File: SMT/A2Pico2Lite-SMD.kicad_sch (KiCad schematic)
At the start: 49 parts, among them J1 SolderJumper_2_Bridged, SW1 SW_BOOTSEL, U1 RP2354A-QFN60, U2 ME6211, X1 ABM8-272-T3 12MHz

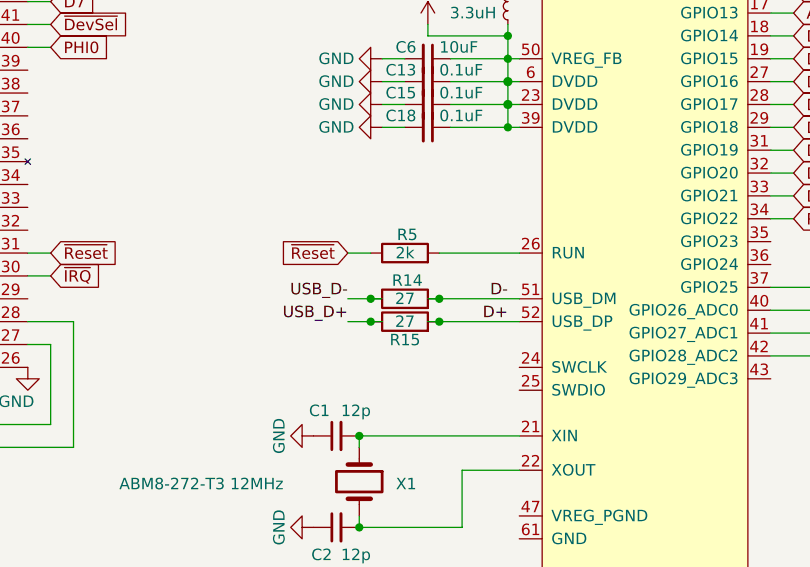
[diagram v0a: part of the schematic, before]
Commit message: Add files via upload
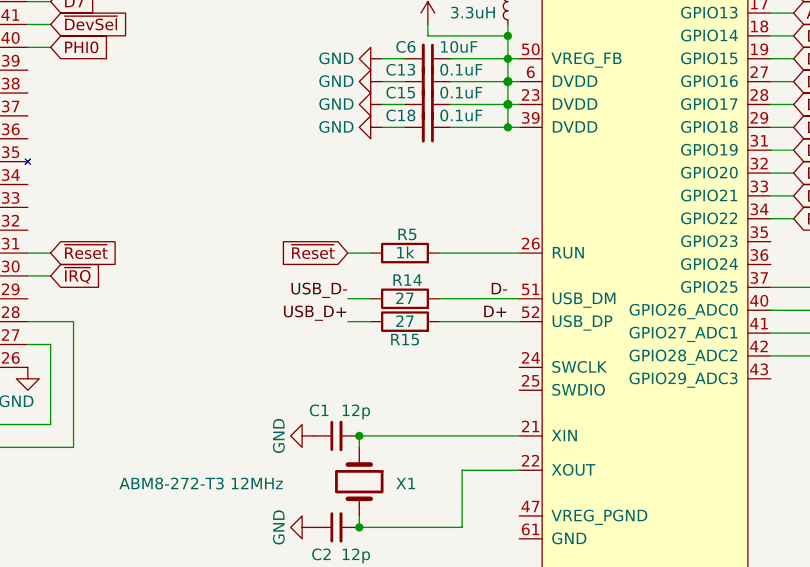
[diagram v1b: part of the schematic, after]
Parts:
- R5: value 2k -> 1k
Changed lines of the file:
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@@
 	)
 	(junction
-		(at 115.57 125.73)
-		(diameter 0)
-		(color 0 0 0 0)
-	)
-	(junction
-		(at 107.95 123.19)
-		(diameter 0)
-		(color 0 0 0 0)
-	)
-	(junction
 		(at 123.19 99.06)
 		(diameter 1.016)
@@
 	)
 	(junction
-		(at 107.95 125.73)
-		(diameter 0)
-		(color 0 0 0 0)
-	)
-	(junction
 		(at 123.19 81.28)
 		(diameter 0)
@@
 	)
 	(junction
-		(at 115.57 123.19)
-		(diameter 0)
-		(color 0 0 0 0)
-	)
-	(junction
 		(at 106.68 138.43)
 		(diameter 0)
@@
 	(wire
 		(pts
+			(xy 115.57 123.19) (xy 124.46 123.19)
+		)
+		(stroke
+			(width 0)
+			(type default)
+		)
+	)
+	(wire
+		(pts
 			(xy 154.94 91.44) (xy 152.4 91.44)
 		)
@@
 	(wire
 		(pts
-			(xy 107.95 125.73) (xy 109.22 125.73)
-		)
-		(stroke
-			(width 0)
-			(type solid)
-		)
-	)
-	(wire
-		(pts
 			(xy 238.76 133.35) (xy 241.3 133.35)
 		)
@@
 	(wire
 		(pts
-			(xy 114.3 123.19) (xy 115.57 123.19)
-		)
-		(stroke
-			(width 0)
-			(type solid)
-		)
-	)
-	(wire
-		(pts
 			(xy 69.85 92.71) (xy 72.39 92.71)
 		)
@@
 	(wire
 		(pts
-			(xy 114.3 125.73) (xy 115.57 125.73)
-		)
-		(stroke
-			(width 0)
-			(type solid)
-		)
-	)
-	(wire
-		(pts
 			(xy 175.26 38.1) (xy 175.26 40.64)
 		)
@@
 	(wire
 		(pts
-			(xy 115.57 123.19) (xy 124.46 123.19)
-		)
-		(stroke
-			(width 0)
-			(type solid)
-		)
-	)
-	(wire
-		(pts
 			(xy 154.94 78.74) (xy 152.4 78.74)
 		)
@@
 	(wire
 		(pts
-			(xy 107.95 123.19) (xy 109.22 123.19)
-		)
-		(stroke
-			(width 0)
-			(type solid)
-		)
-	)
-	(wire
-		(pts
 			(xy 260.35 129.54) (xy 260.35 130.81)
 		)
@@
 			)
 		)
-		(property "Value" "2k"
+		(property "Value" "1k"
 			(at 111.76 118.11 90)
 			(effects
